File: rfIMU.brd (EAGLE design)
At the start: 100 x 80 mm, 0 parts

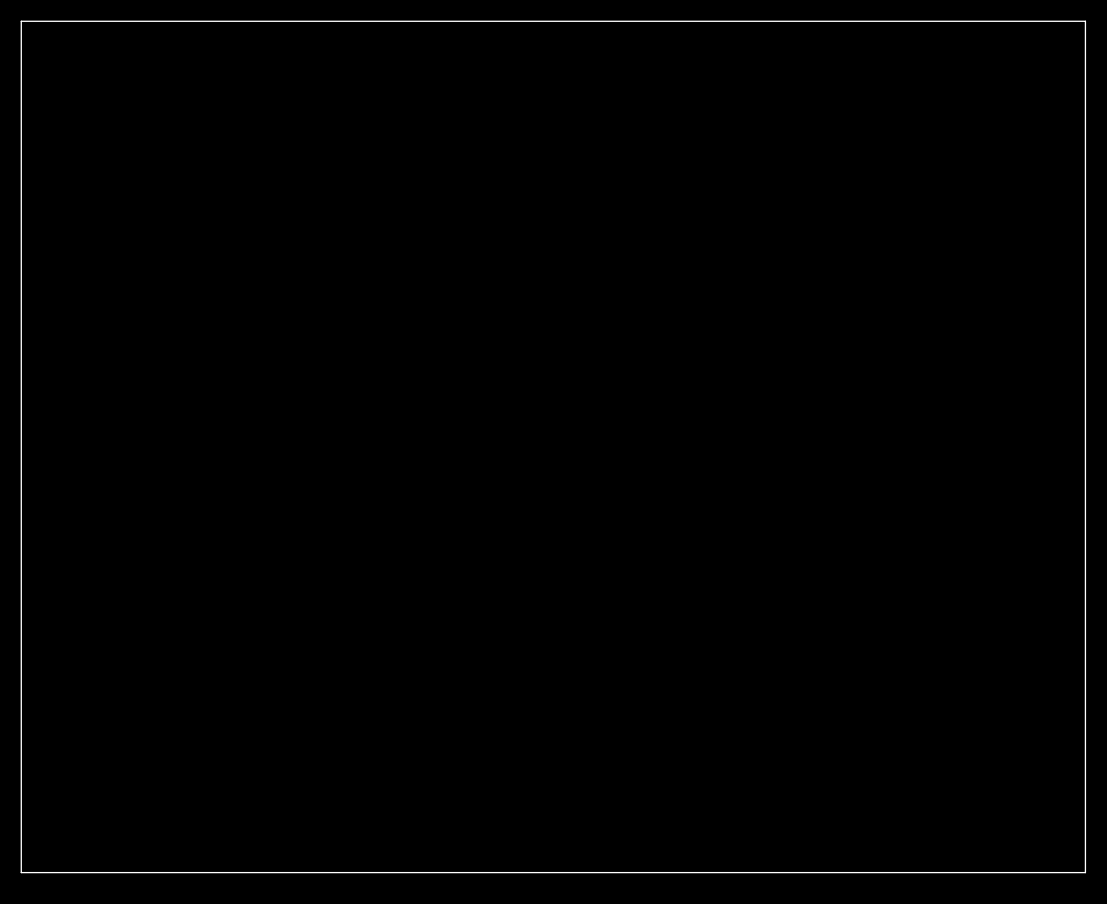
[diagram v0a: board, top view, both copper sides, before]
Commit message: adds v2
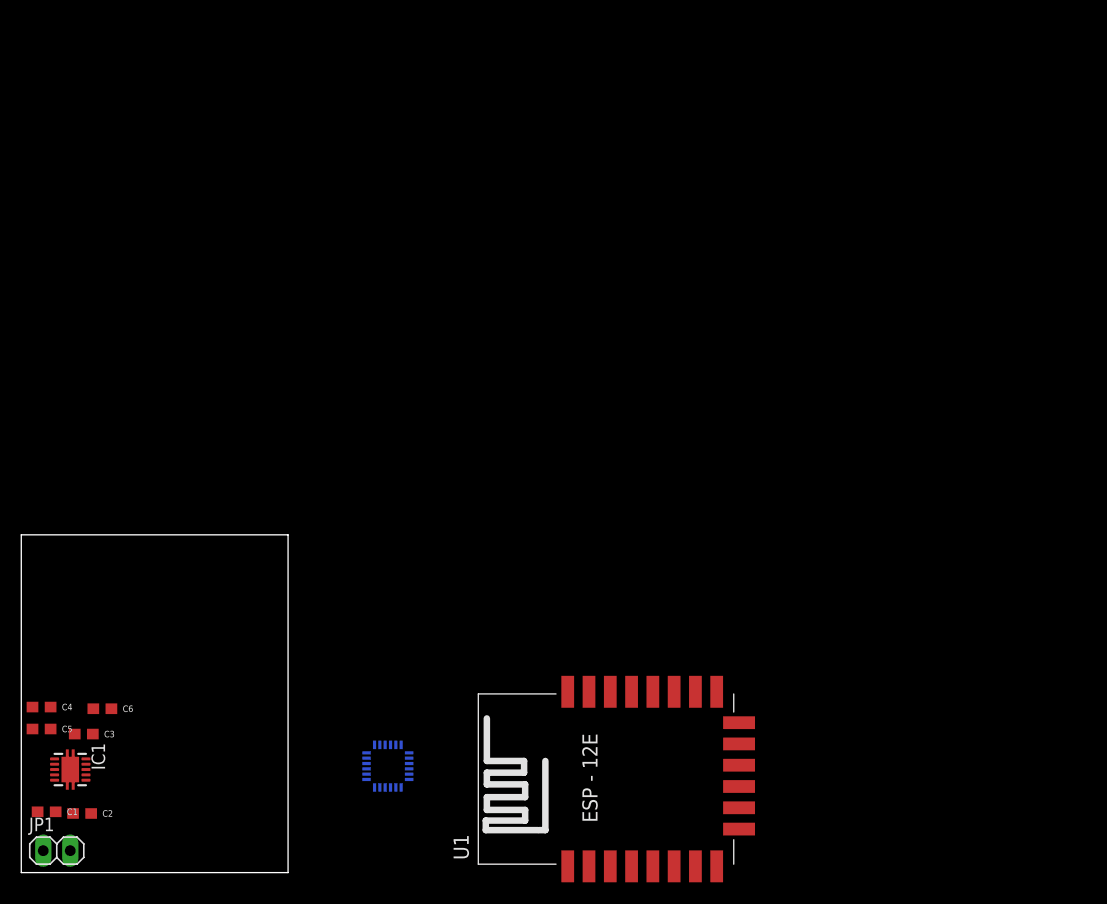
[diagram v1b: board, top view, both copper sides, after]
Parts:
- added C1, C4: 10u, Brendan:0603
- added C2, C3, C6: 0.1u, Brendan:0603
- added C5: 1u, Brendan:0603
- added IC1: TPS61201, texas:S-PDSO-N10
- added JP1: (no value), pinhead:1X02
- added U1: (no value), esp8266modules:ESP12E-SMD
- added U3: (no value), SparkFun-Sensors:QFN-24-NP
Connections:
- new net 3.3V: C1.2, C2.2, C3.2, C4.1, C4.2, C5.1, C5.2, C6.1, C6.2, IC1.10, IC1.2, IC1.4, IC1.8, IC1.9, IC1.PP, IC1.PP@1, IC1.PP@2, U3.15, U3.17, U3.18
- new net N$2: C3.1, IC1.1
- new net N$4: C1.1, C2.1, IC1.5, IC1.6, IC1.7
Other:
- board size 100 x 80 mm -> 25.1 x 31.7 mm
